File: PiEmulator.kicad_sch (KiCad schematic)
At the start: 46 parts, among them J1 Conn_01x01, J2 Conn_01x01, J3 USB_C_Receptacle_USB2.0, U1 ADA3708, U3 BQ24090DGQ, U4 TPS61230DRCR, U5 XD-XH-2AW-G

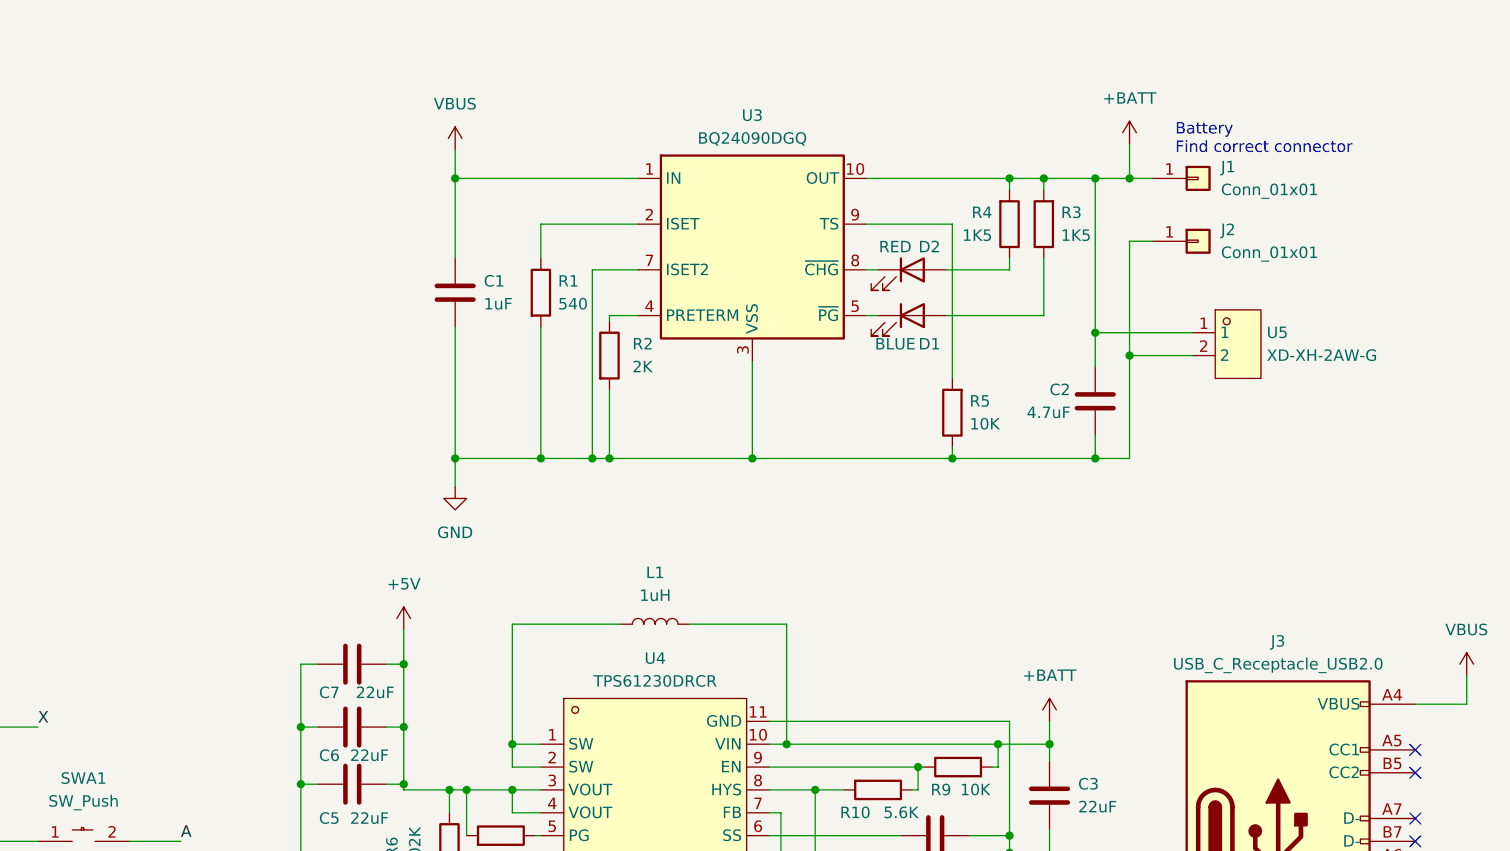
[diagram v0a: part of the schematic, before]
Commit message: added gerbers
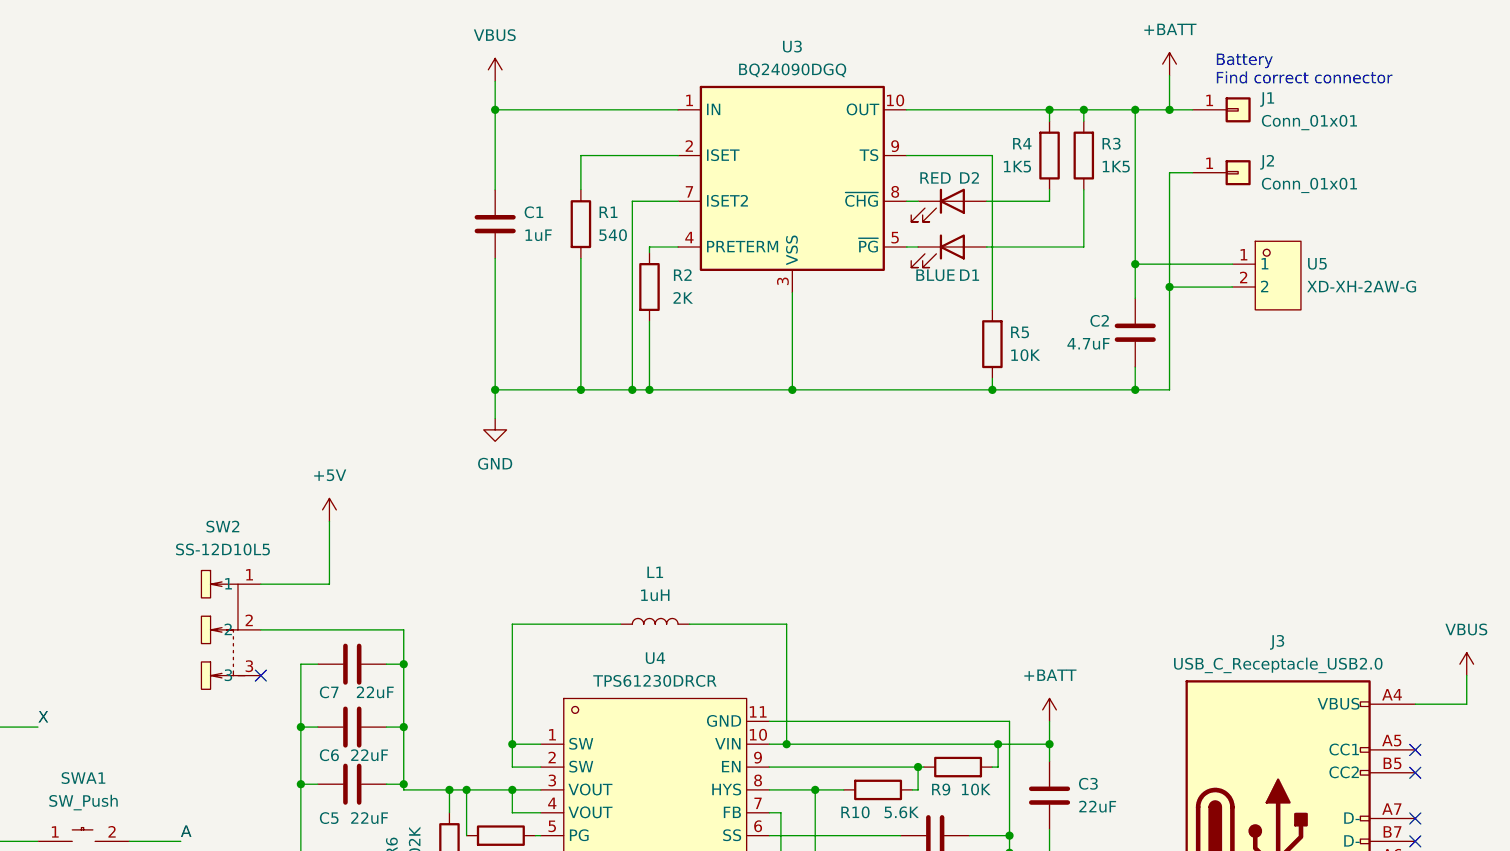
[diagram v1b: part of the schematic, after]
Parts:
- added SW2: SS-12D10L5, easyeda2kicad:SW-TH_SS-12D10L5, symbol easyeda2kicad:SS-12D10L5
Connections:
- net +5V: now also SW2.1; no longer C5.2, C6.2, C7.2, R6.1, R8.2, U4.3 (VOUT), U4.4 (VOUT)
- new net: C5.2, C6.2, C7.2, R6.1, R8.2, SW2.2, U4.3 (VOUT), U4.4 (VOUT)
- no-connect marks 27 -> 28
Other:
- moved on the sheet: C1, C2, D1, D2, J1, J2, R1, R2, R3, R4, R5, U3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
